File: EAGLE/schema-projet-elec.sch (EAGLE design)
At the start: 25 parts

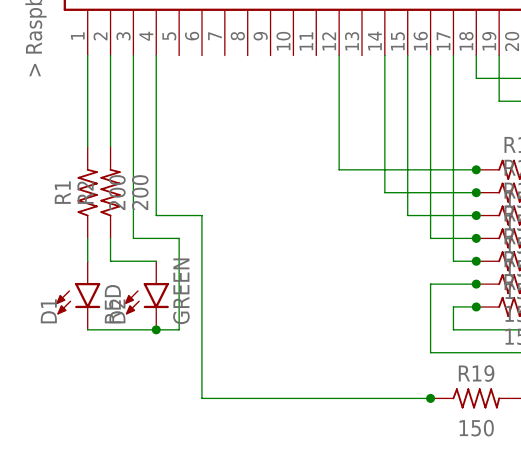
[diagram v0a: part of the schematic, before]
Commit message: Change brd ans sch
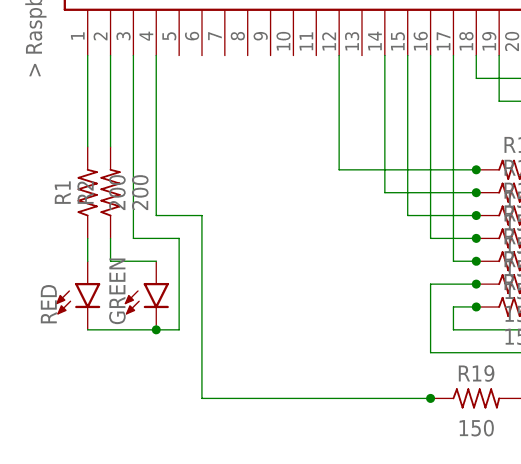
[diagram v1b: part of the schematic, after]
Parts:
- removed D1: RED, SparkFun-LED:LED-RED0603
- removed D2: GREEN, SparkFun-LED:LED-GREEN0603
- added GREEN, RED: (no value), SparkFun-LED:LED5MM
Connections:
- net N$2: now also RED.A; no longer D1.A
- net N$4: now also GREEN.A; no longer D2.A
- net N$5: now also GREEN.C, RED.C; no longer D1.C, D2.C
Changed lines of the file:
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@@
 <part name="R1" library="Resistor" library_urn="urn:adsk.eagle:library:16378527" deviceset="R-US" device="AXIAL-7.2MM-PITCH" package3d_urn="urn:adsk.eagle:package:16378561/2" technology="_" value="200"/>
 <part name="R2" library="Resistor" library_urn="urn:adsk.eagle:library:16378527" deviceset="R-US" device="AXIAL-7.2MM-PITCH" package3d_urn="urn:adsk.eagle:package:16378561/2" technology="_" value="200"/>
-<part name="D1" library="SparkFun-LED" library_urn="urn:adsk.eagle:library:529" deviceset="LED-RED" device="0603" package3d_urn="urn:adsk.eagle:package:39354/1" value="RED"/>
-<part name="D2" library="SparkFun-LED" library_urn="urn:adsk.eagle:library:529" deviceset="LED-GREEN" device="0603" package3d_urn="urn:adsk.eagle:package:39354/1" value="GREEN"/>
 <part name="HC-SR04" library="hc-sr04" deviceset="HC-SR04" device=""/>
 <part name="R3" library="Resistor" library_urn="urn:adsk.eagle:library:16378527" deviceset="R-US" device="AXIAL-7.2MM-PITCH" package3d_urn="urn:adsk.eagle:package:16378561/2" technology="_" value="2000"/>
@@
 <part name="DIS1" library="display-hp" library_urn="urn:adsk.eagle:library:212" deviceset="HD-H103" device="" package3d_urn="urn:adsk.eagle:package:13006/1"/>
 <part name="DIS2" library="display-hp" library_urn="urn:adsk.eagle:library:212" deviceset="HD-H103" device="" package3d_urn="urn:adsk.eagle:package:13006/1"/>
+<part name="RED" library="SparkFun-LED" library_urn="urn:adsk.eagle:library:529" deviceset="LED" device="5MM" package3d_urn="urn:adsk.eagle:package:39353/1"/>
+<part name="GREEN" library="SparkFun-LED" library_urn="urn:adsk.eagle:library:529" deviceset="LED" device="5MM" package3d_urn="urn:adsk.eagle:package:39353/1"/>
 </parts>
 <sheets>
@@
 <attribute name="NAME" x="30.2514" y="33.02" size="1.778" layer="95" rot="R90" align="center"/>
 <attribute name="VALUE" x="36.322" y="33.02" size="1.778" layer="96" rot="R90" align="center"/>
-</instance>
-<instance part="D1" gate="G$1" x="30.48" y="22.86" smashed="yes">
-<attribute name="NAME" x="27.051" y="18.288" size="1.778" layer="95" font="vector" rot="R90"/>
-<attribute name="VALUE" x="32.385" y="18.288" size="1.778" layer="96" font="vector" rot="R90" align="top-left"/>
-</instance>
-<instance part="D2" gate="G$1" x="38.1" y="22.86" smashed="yes">
-<attribute name="NAME" x="34.671" y="18.288" size="1.778" layer="95" font="vector" rot="R90"/>
-<attribute name="VALUE" x="40.005" y="18.288" size="1.778" layer="96" font="vector" rot="R90" align="top-left"/>
 </instance>
 <instance part="HC-SR04" gate="J_ULTRASONIC" x="68.58" y="106.68" smashed="yes">
@@
 <attribute name="VALUE" x="149.86" y="69.85" size="1.778" layer="96" rot="R180"/>
 </instance>
+<instance part="RED" gate="G$1" x="30.48" y="22.86" smashed="yes">
+<attribute name="NAME" x="27.051" y="18.288" size="1.778" layer="95" font="vector" rot="R90"/>
+<attribute name="VALUE" x="32.385" y="18.288" size="1.778" layer="96" font="vector" rot="R90" align="top-left"/>
+</instance>
+<instance part="GREEN" gate="G$1" x="38.1" y="22.86" smashed="yes">
+<attribute name="NAME" x="34.671" y="18.288" size="1.778" layer="95" font="vector" rot="R90"/>
+<attribute name="VALUE" x="40.005" y="18.288" size="1.778" layer="96" font="vector" rot="R90" align="top-left"/>
+</instance>
 </instances>
 <busses>
@@
 <segment>
 <pinref part="R1" gate="G$1" pin="1"/>
-<pinref part="D1" gate="G$1" pin="A"/>
 <wire x1="30.48" y1="27.94" x2="30.48" y2="25.4" width="0.1524" layer="91"/>
+<pinref part="RED" gate="G$1" pin="A"/>
 </segment>
 </net>
@@
 <segment>
 <pinref part="R2" gate="G$1" pin="1"/>
-<pinref part="D2" gate="G$1" pin="A"/>
 <wire x1="33.02" y1="27.94" x2="33.02" y2="25.4" width="0.1524" layer="91"/>
 <wire x1="33.02" y1="25.4" x2="38.1" y2="25.4" width="0.1524" layer="91"/>
+<pinref part="GREEN" gate="G$1" pin="A"/>
 </segment>
 </net>
 <net name="N$5" class="0">
 <segment>
-<pinref part="D2" gate="G$1" pin="C"/>
-<wire x1="38.1" y1="17.78" x2="40.64" y2="17.78" width="0.1524" layer="91"/>
 <wire x1="40.64" y1="17.78" x2="40.64" y2="27.94" width="0.1524" layer="91"/>
 <pinref part="U$1" gate="G$1" pin="3"/>
 <wire x1="40.64" y1="27.94" x2="35.56" y2="27.94" width="0.1524" layer="91"/>
 <wire x1="35.56" y1="27.94" x2="35.56" y2="48.26" width="0.1524" layer="91"/>
-<pinref part="D1" gate="G$1" pin="C"/>
 <wire x1="30.48" y1="17.78" x2="38.1" y2="17.78" width="0.1524" layer="91"/>
+<pinref part="RED" gate="G$1" pin="C"/>
+<pinref part="GREEN" gate="G$1" pin="C"/>
+<wire x1="38.1" y1="17.78" x2="40.64" y2="17.78" width="0.1524" layer="91"/>
 <junction x="38.1" y="17.78"/>
 </segment>

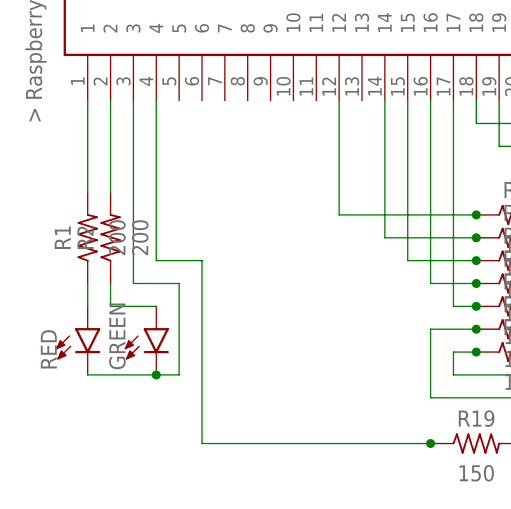
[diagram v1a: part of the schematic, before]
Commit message: Add files via upload
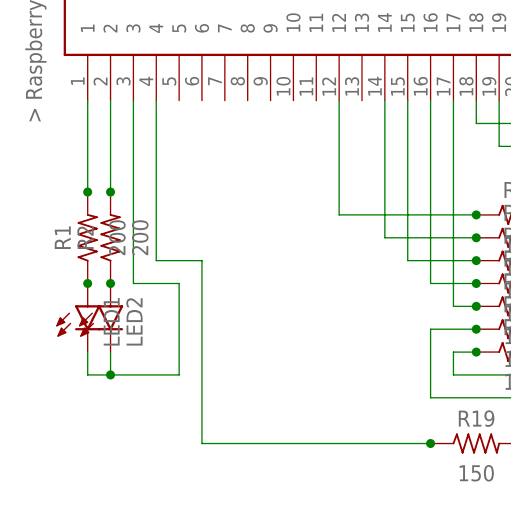
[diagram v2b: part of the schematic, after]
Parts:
- removed GREEN, RED: (no value), SparkFun-LED:LED5MM
- added LED1, LED2: (no value), led:LED5MM
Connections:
- net N$2: now also LED1.A; no longer RED.A
- net N$4: now also LED2.A; no longer GREEN.A
- net N$5: now also LED1.C, LED2.C; no longer GREEN.C, RED.C
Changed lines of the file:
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@@
 <part name="DIS1" library="display-hp" library_urn="urn:adsk.eagle:library:212" deviceset="HD-H103" device="" package3d_urn="urn:adsk.eagle:package:13006/1"/>
 <part name="DIS2" library="display-hp" library_urn="urn:adsk.eagle:library:212" deviceset="HD-H103" device="" package3d_urn="urn:adsk.eagle:package:13006/1"/>
-<part name="RED" library="SparkFun-LED" library_urn="urn:adsk.eagle:library:529" deviceset="LED" device="5MM" package3d_urn="urn:adsk.eagle:package:39353/1"/>
-<part name="GREEN" library="SparkFun-LED" library_urn="urn:adsk.eagle:library:529" deviceset="LED" device="5MM" package3d_urn="urn:adsk.eagle:package:39353/1"/>
+<part name="LED1" library="led" library_urn="urn:adsk.eagle:library:259" deviceset="LED" device="5MM" package3d_urn="urn:adsk.eagle:package:15799/2"/>
+<part name="LED2" library="led" library_urn="urn:adsk.eagle:library:259" deviceset="LED" device="5MM" package3d_urn="urn:adsk.eagle:package:15799/2"/>
 </parts>
 <sheets>
@@
 <attribute name="VALUE" x="149.86" y="69.85" size="1.778" layer="96" rot="R180"/>
 </instance>
-<instance part="RED" gate="G$1" x="30.48" y="22.86" smashed="yes">
-<attribute name="NAME" x="27.051" y="18.288" size="1.778" layer="95" font="vector" rot="R90"/>
-<attribute name="VALUE" x="32.385" y="18.288" size="1.778" layer="96" font="vector" rot="R90" align="top-left"/>
-</instance>
-<instance part="GREEN" gate="G$1" x="38.1" y="22.86" smashed="yes">
-<attribute name="NAME" x="34.671" y="18.288" size="1.778" layer="95" font="vector" rot="R90"/>
-<attribute name="VALUE" x="40.005" y="18.288" size="1.778" layer="96" font="vector" rot="R90" align="top-left"/>
+<instance part="LED1" gate="G$1" x="30.48" y="25.4" smashed="yes">
+<attribute name="NAME" x="34.036" y="20.828" size="1.778" layer="95" rot="R90"/>
+<attribute name="VALUE" x="36.195" y="20.828" size="1.778" layer="96" rot="R90"/>
+</instance>
+<instance part="LED2" gate="G$1" x="33.02" y="25.4" smashed="yes">
+<attribute name="NAME" x="36.576" y="20.828" size="1.778" layer="95" rot="R90"/>
+<attribute name="VALUE" x="38.735" y="20.828" size="1.778" layer="96" rot="R90"/>
 </instance>
 </instances>
@@
 <pinref part="R1" gate="G$1" pin="2"/>
 <wire x1="30.48" y1="48.26" x2="30.48" y2="38.1" width="0.1524" layer="91"/>
-</segment>
-</net>
-<net name="N$2" class="0">
-<segment>
-<pinref part="R1" gate="G$1" pin="1"/>
-<wire x1="30.48" y1="27.94" x2="30.48" y2="25.4" width="0.1524" layer="91"/>
-<pinref part="RED" gate="G$1" pin="A"/>
+<junction x="30.48" y="38.1"/>
 </segment>
 </net>
@@
 <pinref part="R2" gate="G$1" pin="2"/>
 <wire x1="33.02" y1="48.26" x2="33.02" y2="38.1" width="0.1524" layer="91"/>
-</segment>
-</net>
-<net name="N$4" class="0">
-<segment>
-<pinref part="R2" gate="G$1" pin="1"/>
-<wire x1="33.02" y1="27.94" x2="33.02" y2="25.4" width="0.1524" layer="91"/>
-<wire x1="33.02" y1="25.4" x2="38.1" y2="25.4" width="0.1524" layer="91"/>
-<pinref part="GREEN" gate="G$1" pin="A"/>
+<junction x="33.02" y="38.1"/>
 </segment>
 </net>
 <net name="N$5" class="0">
 <segment>
-<wire x1="40.64" y1="17.78" x2="40.64" y2="27.94" width="0.1524" layer="91"/>
 <pinref part="U$1" gate="G$1" pin="3"/>
-<wire x1="40.64" y1="27.94" x2="35.56" y2="27.94" width="0.1524" layer="91"/>
 <wire x1="35.56" y1="27.94" x2="35.56" y2="48.26" width="0.1524" layer="91"/>
-<wire x1="30.48" y1="17.78" x2="38.1" y2="17.78" width="0.1524" layer="91"/>
-<pinref part="RED" gate="G$1" pin="C"/>
-<pinref part="GREEN" gate="G$1" pin="C"/>
-<wire x1="38.1" y1="17.78" x2="40.64" y2="17.78" width="0.1524" layer="91"/>
-<junction x="38.1" y="17.78"/>
+<wire x1="35.56" y1="27.94" x2="40.64" y2="27.94" width="0.1524" layer="91"/>
+<wire x1="40.64" y1="27.94" x2="40.64" y2="17.78" width="0.1524" layer="91"/>
+<wire x1="40.64" y1="17.78" x2="33.02" y2="17.78" width="0.1524" layer="91"/>
+<pinref part="LED1" gate="G$1" pin="C"/>
+<wire x1="33.02" y1="17.78" x2="30.48" y2="17.78" width="0.1524" layer="91"/>
+<wire x1="30.48" y1="17.78" x2="30.48" y2="20.32" width="0.1524" layer="91"/>
+<pinref part="LED2" gate="G$1" pin="C"/>
+<wire x1="33.02" y1="20.32" x2="33.02" y2="17.78" width="0.1524" layer="91"/>
+<junction x="33.02" y="17.78"/>
 </segment>
 </net>
@@
 </segment>
 </net>
+<net name="N$2" class="0">
+<segment>
+<pinref part="R1" gate="G$1" pin="1"/>
+<pinref part="LED1" gate="G$1" pin="A"/>
+<junction x="30.48" y="27.94"/>
+</segment>
+</net>
+<net name="N$4" class="0">
+<segment>
+<pinref part="R2" gate="G$1" pin="1"/>
+<pinref part="LED2" gate="G$1" pin="A"/>
+<junction x="33.02" y="27.94"/>
+</segment>
+</net>
